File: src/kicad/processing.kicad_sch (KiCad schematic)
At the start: 46 parts, among them J1 SD_Card_Receptacle, J4 Conn_01x03, SW11 SW_Push, U1 ABM8-272-T3_C20625731, U2 FSC-BT1114QI, U3 W25Q128JVE, U4 APS6404L-SQRx-ZR, U6 RP2350B

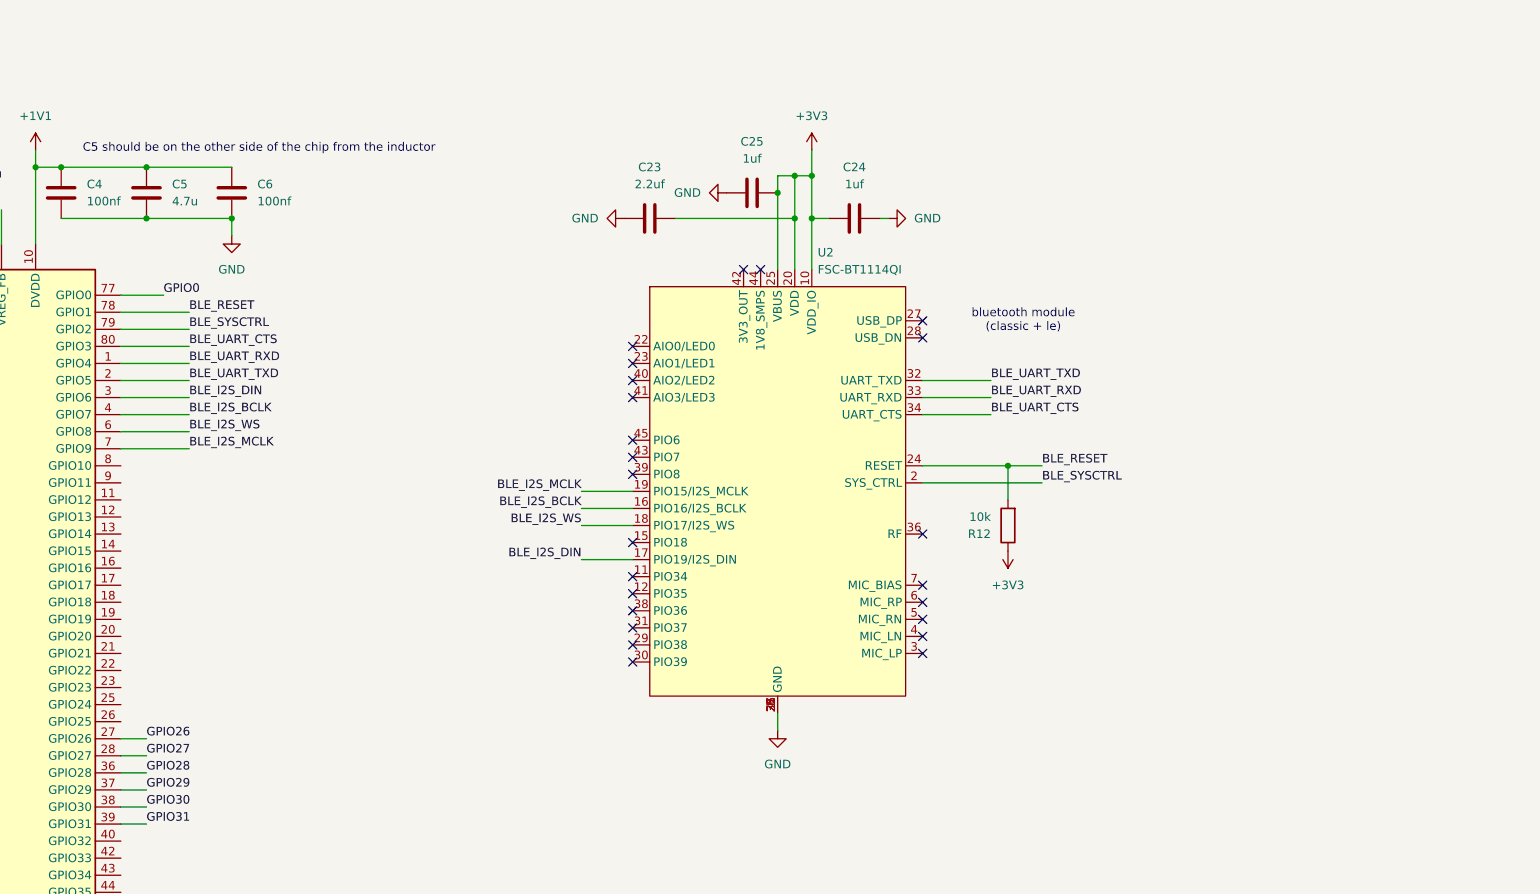
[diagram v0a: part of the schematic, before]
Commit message: new journal entry!
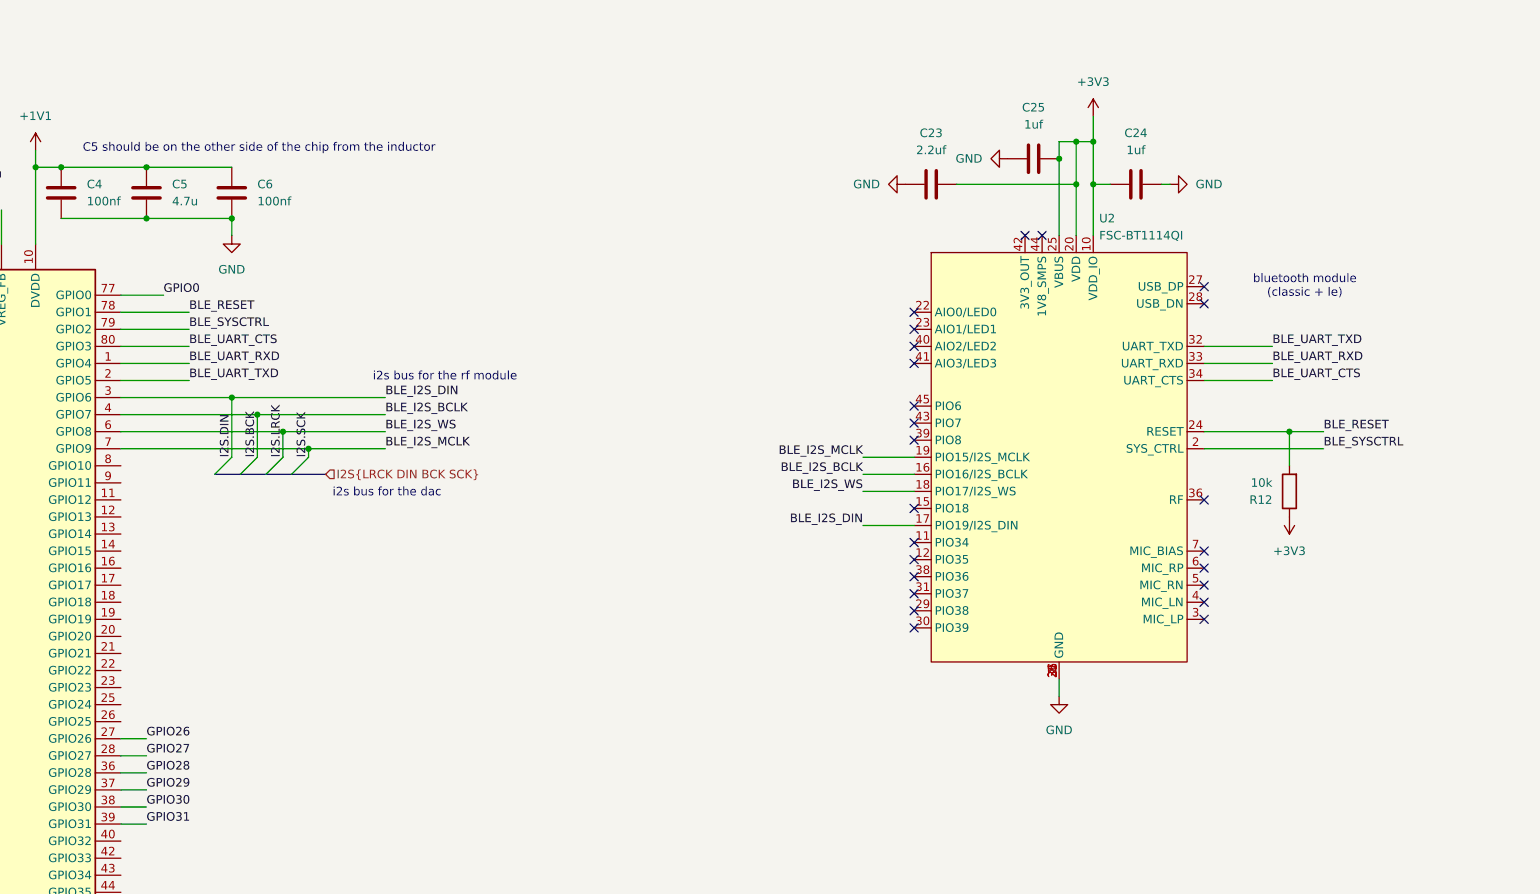
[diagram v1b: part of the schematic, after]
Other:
- note added: "i2s bus for the dac"
- note added: "i2s bus for the rf module"
- moved on the sheet: C23, C24, C25, R12, U2

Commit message: progress + new journal entry!
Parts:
- added C53: 4.7uf, symbol Device:C
- added C54: 200nf, symbol Device:C
- added C55: 1uf, symbol Device:C
- added D1: D, symbol Device:D
- added J6: Conn_01x40, symbol Connector_Generic:Conn_01x40
- added L3: 10uh, symbol Device:L
- added R34: 5, symbol Device:R
- added R35, R47: 10k, symbol Device:R
- added R36, R37: 4.7k, symbol Device:R
- added U11: TPS61165DRV, Package_SON:WSON-6-1EP_2x2mm_P0.65mm_EP1x1.6mm, symbol Driver_LED:TPS61165DRV
- added U12: TCA9555RTWR, Package_DFN_QFN:WQFN-24-1EP_4x4mm_P0.5mm_EP2.45x2.45mm, symbol Interface_Expansion:TCA9555RTWR
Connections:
- net +3V3: now also J6.36 (Pin_36), R35.2, R36.2, R37.2, R47.1, U12.21 (VCC)
- net GND: now also C53.1, C54.2, C55.1, J6.1 (Pin_1), J6.37 (Pin_37), J6.7 (Pin_7), R34.2, U11.3 (GND), U11.7 (GND), U12.18 (A0), U12.23 (A1), U12.24 (A2), U12.25 (EPAD), U12.9 (GND)
- net GPIO26: now also U6.56 (GPIO45/ADC5); no longer U6.27 (GPIO26)
- net GPIO27: now also U6.55 (GPIO44/ADC4); no longer U6.28 (GPIO27)
- net GPIO28: now also U6.54 (GPIO43/ADC3); no longer U6.36 (GPIO28)
- net GPIO29: now also U6.53 (GPIO42/ADC2); no longer U6.37 (GPIO29)
- net GPIO30: now also U6.52 (GPIO41/ADC1); no longer U6.38 (GPIO30)
- net GPIO31: now also U6.49 (GPIO40/ADC0); no longer U6.39 (GPIO31)
- net CARD_DETECT: now reaches J1.10 (CARD_DETECT)
- net CARD_DETECT: now also R47.2, U12.4 (P03)
- net SCREEN_DIMMING: now reaches U6.11 (GPIO12)
- net SCREEN_DIMMING: now also U11.5 (CTRL)
- net SPI.CS: now reaches U6.12 (GPIO13)
- net SPI.CS: now also J6.30 (Pin_30)
- net SPI.SCK: now reaches U6.13 (GPIO14)
- net SPI.SCK: now also J6.31 (Pin_31)
- net SPI.SDA: now reaches U6.14 (GPIO15)
- net SPI.SDA: now also J6.32 (Pin_32)
- net SPI.PCLK: now reaches U6.16 (GPIO16)
- net SPI.PCLK: now also J6.29 (Pin_29)
- net SPI.DE: now reaches U6.17 (GPIO17)
- net SPI.DE: now also J6.28 (Pin_28)
- net SPI.VS: now reaches U6.18 (GPIO18)
- net SPI.VS: now also J6.27 (Pin_27)
- net SPI.HS: now reaches U6.19 (GPIO19)
- net SPI.HS: now also J6.26 (Pin_26)
- net DB0: now reaches U6.20 (GPIO20)
- net DB0: now also J6.25 (Pin_25)
- net DB1: now reaches U6.21 (GPIO21)
- net DB1: now also J6.24 (Pin_24)
- net DB2: now reaches U6.22 (GPIO22)
- net DB2: now also J6.23 (Pin_23)
- net DB3: now reaches U6.23 (GPIO23)
- net DB3: now also J6.22 (Pin_22)
- net DB4: now reaches U6.25 (GPIO24)
- net DB4: now also J6.21 (Pin_21)
- net DB5: now reaches U6.26 (GPIO25)
- net DB5: now also J6.20 (Pin_20)
- net DB12: now reaches U6.40 (GPIO32)
- net DB12: now also J6.13 (Pin_13)
- net DB13: now reaches U6.42 (GPIO33)
- net DB13: now also J6.12 (Pin_12)
- net DB14: now reaches U6.43 (GPIO34)
- net DB14: now also J6.11 (Pin_11)
- net DB15: now reaches U6.44 (GPIO35)
- net DB15: now also J6.10 (Pin_10)
- net DB16: now reaches U6.45 (GPIO36)
- net DB16: now also J6.9 (Pin_9)
- net DB17: now reaches U6.46 (GPIO37)
- net DB17: now also J6.8 (Pin_8)
- net BAT_SOC_SDA: now reaches U6.47 (GPIO38)
- net BAT_SOC_SDA: now also R36.1, U12.20 (SDA)
- net BAT_SOC_SCL: now reaches U6.48 (GPIO39)
- net BAT_SOC_SCL: now also R37.1, U12.19 (SCL)
- net POWER_GPIO: now reaches U6.8 (GPIO10)
- new net: D1.2 (A), L3.2, U11.4 (SW)
- new net: C54.1, U11.2 (COMP)
- new net ANALOG_LDO_EN: U12.3 (P02)
- new net DB10: J6.15 (Pin_15), U6.38 (GPIO30)
- new net DB11: J6.14 (Pin_14), U6.39 (GPIO31)
- new net DB6: J6.19 (Pin_19), U6.27 (GPIO26)
- new net DB7: J6.18 (Pin_18), U6.28 (GPIO27)
- new net DB8: J6.17 (Pin_17), U6.36 (GPIO28)
- new net DB9: J6.16 (Pin_16), U6.37 (GPIO29)
- new net DISPLAY_RESET: J6.35 (Pin_35)
- new net DPAD.CENTER: U12.17 (P17)
- new net DPAD.DOWN: U12.14 (P14)
- new net DPAD.LEFT: U12.15 (P15)
- new net DPAD.RIGHT: U12.16 (P16)
- new net DPAD.UP: U12.13 (P13)
- new net EXPANDER_INT: R35.1, U12.22 (~{INT})
- new net JACK_DETECTION: U12.2 (P01)
- new net LED_A: C55.2, D1.1 (K), J6.40 (Pin_40)
- new net LED_K: J6.38 (Pin_38), J6.39 (Pin_39), R34.1, U11.1 (FB)
- new net POWER_BTN_SENSE: U12.1 (P00)
- new net SCREEN_POWER: C53.2, L3.1, U11.6 (VIN)
- new net VOLUME.DOWN: U12.12 (P12)
- new net VOLUME.UP: U12.11 (P11)
- no-connect marks 24 -> 31
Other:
- note added: "screen backlight power supply"
- note added: "screen connector"
- note added: "touch related pins"
- note removed: "connect card_detect to a gpio later"
- note removed: "processing unit"
- moved on the sheet: C10, C11, C12, C13, C14, C15, C22, C23, C24, C25, C4, C5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

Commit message: may 28th
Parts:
- added R29: 10k, Resistor_SMD:R_0402_1005Metric, symbol Device:R
- R10, R11, R12, R35, R47, R5, R7, R8, R9: footprint (none) -> Resistor_SMD:R_0402_1005Metric
- R34: footprint (none) -> Resistor_SMD:R_0603_1608Metric; LCSC Part (none) -> C25197; Tolerance (none) -> 1%
- R36, R37: footprint (none) -> Resistor_SMD:R_0402_1005Metric; LCSC Part (none) -> C25900
- SW11: value SW_Push -> TS-1088-AR02016; footprint (none) -> easyeda2kicad:SW-SMD_L3.9-W3.0-P4.45; LCSC Part (none) -> C720477
- U11: LCSC Part (none) -> C122568
- U12: LCSC Part (none) -> C140277
- U2: footprint (none) -> feasycom:FSC-BT1114QI
- U3: LCSC Part (none) -> C2456297
- U4: LCSC Part (none) -> C3040877
- U6: LCSC Part (none) -> C42415655
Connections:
- net +3V3: now also R29.1
- net CHG_PIN: now reaches U12.7 (P06)
- net CHG_PIN: now also R29.2
